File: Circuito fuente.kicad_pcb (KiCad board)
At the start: 2 copper layers, 99.1 x 99 mm, 37 parts, among them Q1 TIP122, U1 Bornera_1x3, U2 Bornera_1x2, U3 Bornera_1x3, U35 LM7812_TO220, U39 LM7912_TO220, U4 LM7812_TO220, U40 LM7805_TO220, U41 LM7905_TO220, U45 LD1117S12TR_SOT223, U5 Bornera_1x3, U6 Bornera_1x2

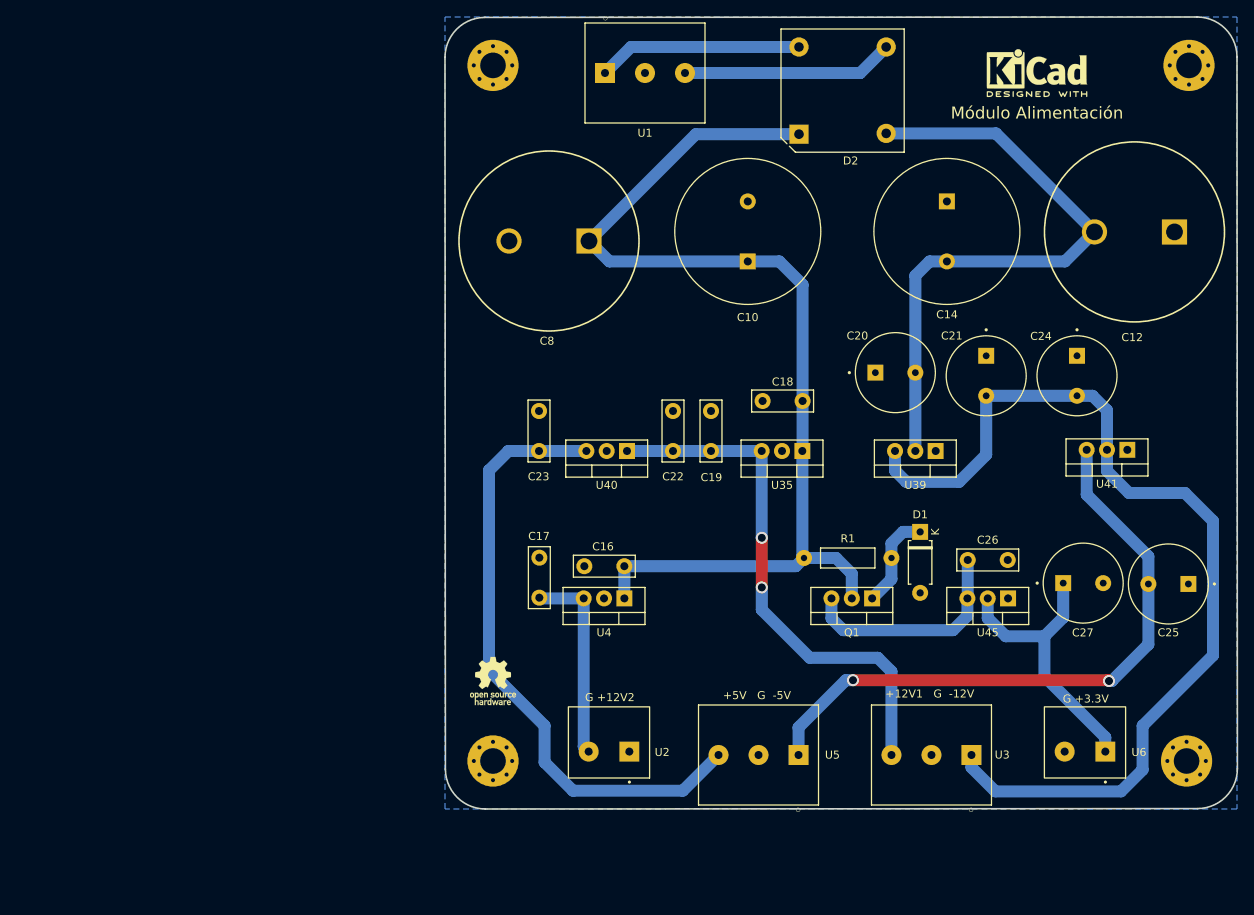
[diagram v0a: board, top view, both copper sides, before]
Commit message: Last version
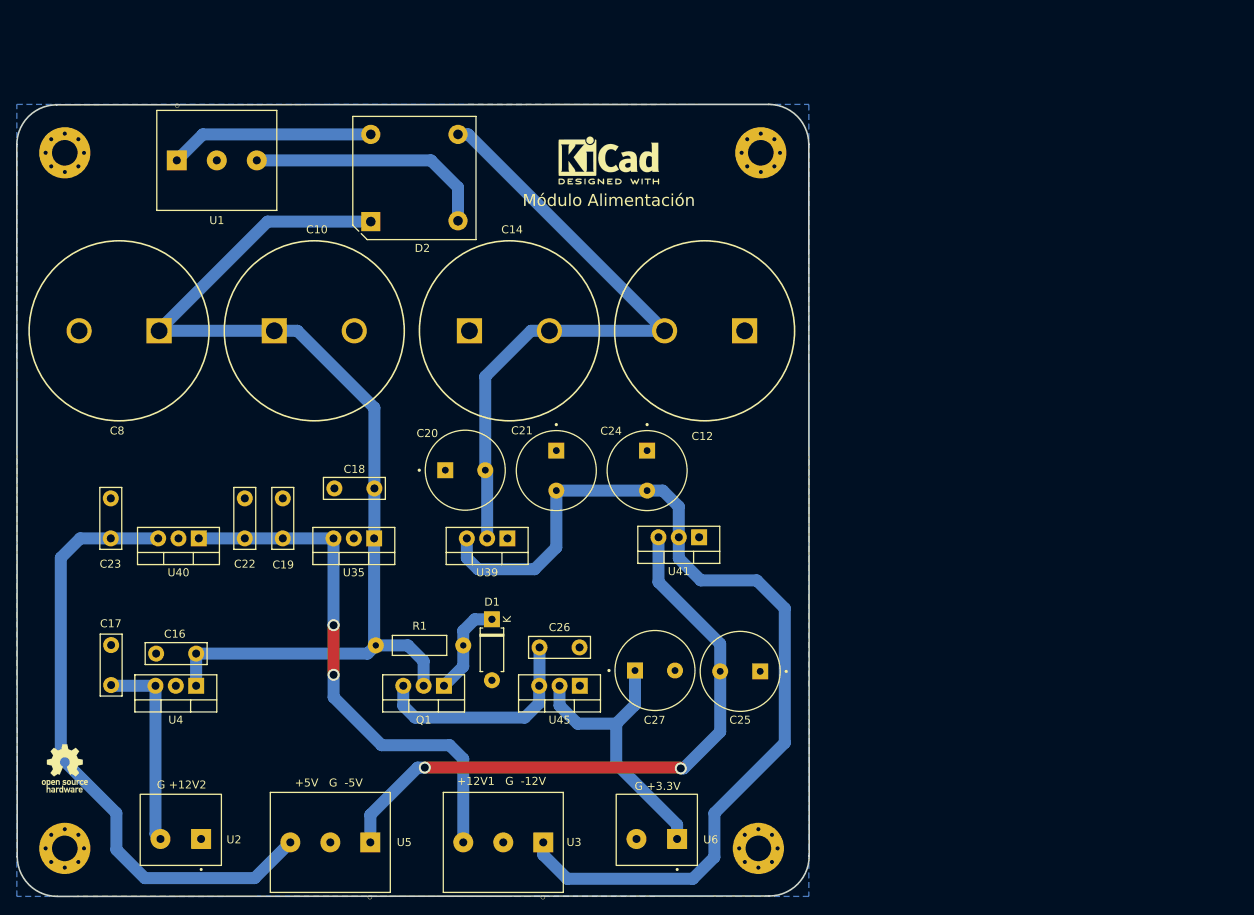
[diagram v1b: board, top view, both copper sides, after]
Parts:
- C10, C14: footprint CEDCp:Cap_4700uF_35V -> CEDCp:Cap_4700uF_50V
- moved C14 61.8 mm to (101.1, 67.7), turned to 0 degrees
- moved C10 59.8 mm to (76.7, 67.7), turned to 0 degrees
- moved C12 55.1 mm to (135.4, 67.7)
- moved C20 55.1 mm to (100.5, 85.2)
- moved C21 55.0 mm to (111.9, 85.2)
- moved C24 55.0 mm to (123.3, 85.2)
- moved C8 54.9 mm to (62.3, 67.7)
- moved C26 54.6 mm to (109.8, 107.3)
- moved R1 54.6 mm to (94.8, 107.0)
- moved U3 54.6 mm to (105.3, 131.7)
- moved U39 54.6 mm to (105.8, 93.7)
- moved C16 54.6 mm to (66.9, 108.1)
- moved C19 54.6 mm to (77.7, 93.7)
- moved C22 54.6 mm to (73.0, 93.7)
- moved C25 54.6 mm to (134.9, 110.3)
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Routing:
- net /+15VAC: track 26.5 -> 30.7 mm
- net Net-(C12-Pad2): track 77.7 -> 81.1 mm
- net /+15DC: track 131.8 -> 129.6 mm
- net /-12V: track 122.5 -> 121.0 mm
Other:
- outline, holes or cut-outs redrawn
